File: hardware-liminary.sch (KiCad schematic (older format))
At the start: 51 parts, among them J1 Conn_01x05, J2 Conn_01x03, J3 Conn_01x03, J4 Conn_02x05_Odd_Even, J5 Conn_01x02, J6 UFL Conn, K1 HL2-1CH-12S, Q1 CMBT3904, Q2 PT204-6C, Q3 CMBT2222A, SW1 SW_Push, U1 EESAMR34J18-V1_CT, U2 LD1117S33TR_SOT223, U6 MCP6001T-I_OT

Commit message: eesam34
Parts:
- removed J6: UFL Conn, symbol 1909763-1:1909763-1
- removed LED1: 12-22/G6R6C-A31/2C, symbol LED_12-22:12-22SURSYGC_S530-A2_TR8
- removed U1: EESAMR34J18-V1_CT, symbol EESAMR34:EESAMR34J18-V1_CT
- removed U6: MCP6001T-I_OT, symbol MCP6001T-I_OT:MCP6001T-I_OT
- added U1: EESAMR34J18-V1_CT, proyect_EESAMR34:EESAMR34, symbol proyect_EESAMR34J18-V1_CT:EESAMR34J18-V1_CT
- JP3, JP4: footprint (none) -> Resistor_SMD:R_1206_3216Metric_Pad1.42x1.75mm_HandSolder
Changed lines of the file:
@@
 	3100 1350 3100 1250
-$Comp
-L MCP6001T-I_OT:MCP6001T-I_OT U6
-U 1 1 5F764C68
-P 3550 3500
-F 0 "U6" H 4150 3350 50  0000 C CNN
-F 1 "MCP6001T-I_OT" H 4150 3250 50  0000 C CNN
-F 2 "" H 4600 3900 50  0001 L CNN
-F 3 "http://docs-emea.rs-online.com/webdocs/0dd1/0900766b80dd189c.pdf" H 4600 3800 50  0001 L CNN
-F 4 "Single 1.8V Op Amp, 1MHz, I temp" H 4600 3700 50  0001 L CNN "Description"
-F 5 "1.45" H 4600 3600 50  0001 L CNN "Height"
-F 6 "Microchip" H 4600 3500 50  0001 L CNN "Manufacturer_Name"
-F 7 "MCP6001T-I/OT" H 4600 3400 50  0001 L CNN "Manufacturer_Part_Number"
-F 8 "MCP6001T-I/OT" H 4600 3300 50  0001 L CNN "Arrow Part Number"
-F 9 "https://www.arrow.com/en/products/mcp6001t-iot/microchip-technology" H 4600 3200 50  0001 L CNN "Arrow Price/Stock"
-F 10 "579-MCP6001T-I/OT" H 4600 3100 50  0001 L CNN "Mouser Part Number"
-F 11 "https://www.mouser.co.uk/ProductDetail/Microchip-Technology/MCP6001T-I-OT?qs=Q%2Fw7XRh99iki9dglS7IqJg%3D%3D" H 4600 3000 50  0001 L CNN "Mouser Price/Stock"
-	1    3550 3500
-	-1   0    0    -1
-$EndComp
 $Comp
 L Device:R R7
@@
 Wire Notes Line
 	5800 2400 500  2400
-$Comp
-L EESAMR34:EESAMR34J18-V1_CT U1
-U 1 1 5F95A58C
-P 2000 6650
-F 0 "U1" H 2150 6700 50  0000 R CNN
-F 1 "EESAMR34J18-V1_CT" H 2500 6550 50  0000 R CNN
-F 2 "" H 2000 6650 50  0001 L BNN
-F 3 "" H 2000 6650 118 0001 C CNN
-	1    2000 6650
-	1    0    0    -1
-$EndComp
 $Comp
 L power:GNDD #PWR0103
@@
 	1800 7650 1800 8150
 $Comp
-L LED_12-22:12-22SURSYGC_S530-A2_TR8 LED1
-U 1 1 5F8C80DF
-P 4500 8150
-F 0 "LED1" H 5000 8415 50  0000 C CNN
-F 1 "12-22/G6R6C-A31/2C" H 5000 8324 50  0000 C CNN
-F 2 "" H 5350 8250 50  0001 L CNN
-F 3 "" H 5350 8150 50  0001 L CNN
-F 4 "" H 5350 8050 50  0001 L CNN "Description"
-F 5 "2.2" H 5350 7950 50  0001 L CNN "Height"
-F 6 "Everlight" H 5350 7850 50  0001 L CNN "Manufacturer_Name"
-F 7 "12-22SURSYGC/S530-A2/TR8" H 5350 7750 50  0001 L CNN "Manufacturer_Part_Number"
-F 8 "12-22SURSYGC/S530-A2/TR8" H 5350 7650 50  0001 L CNN "Arrow Part Number"
-F 9 "" H 5350 7550 50  0001 L CNN "Arrow Price/Stock"
-F 10 "638-1222SURSYGCA2TR8" H 5350 7450 50  0001 L CNN "Mouser Part Number"
-F 11 "https://www.mouser.com/Search/Refine.aspx?Keyword=638-1222SURSYGCA2TR8" H 5350 7350 50  0001 L CNN "Mouser Price/Stock"
-	1    4500 8150
-	-1   0    0    -1
-$EndComp
-$Comp
 L Device:R R11
 U 1 1 5F8CC602
@@
 Antenna
 $Comp
-L 1909763-1:1909763-1 J6
-U 1 1 5FA17C3E
-P 6900 6000
-F 0 "J6" H 7188 6040 50  0000 L CNN
-F 1 "UFL Conn" H 7188 5949 50  0000 L CNN
-F 2 "" H 6900 6000 50  0001 L BNN
-F 3 "1909763-1" H 6900 6000 50  0001 L BNN
-F 4 "1" H 6900 6000 50  0001 L BNN "Field4"
-	1    6900 6000
-	1    0    0    -1
-$EndComp
-$Comp
 L power:GNDD #PWR014
 U 1 1 5FA23786
@@
 F 0 "JP4" H 6400 6164 50  0000 C CNN
 F 1 "Jumper" H 6400 6073 50  0000 C CNN
-F 2 "" H 6400 5900 50  0001 C CNN
+F 2 "Resistor_SMD:R_1206_3216Metric_Pad1.42x1.75mm_HandSolder" H 6400 5900 50  0001 C CNN
 F 3 "~" H 6400 5900 50  0001 C CNN
 	1    6400 5900
@@
 F 0 "JP3" H 6400 5814 50  0000 C CNN
 F 1 "Jumper" H 6400 5723 50  0000 C CNN
-F 2 "" H 6400 5550 50  0001 C CNN
+F 2 "Resistor_SMD:R_1206_3216Metric_Pad1.42x1.75mm_HandSolder" H 6400 5550 50  0001 C CNN
 F 3 "~" H 6400 5550 50  0001 C CNN
 	1    6400 5550
@@
 Wire Notes Line
 	7750 2350 7750 500
+$Comp
+L proyect_EESAMR34J18-V1_CT:EESAMR34J18-V1_CT U1
+U 1 1 5F767C93
+P 2000 6650
+F 0 "U1" H 1057 6646 50  0000 R CNN
+F 1 "EESAMR34J18-V1_CT" H 1057 6555 50  0000 R CNN
+F 2 "proyect_EESAMR34:EESAMR34" H 2000 6650 50  0001 L BNN
+F 3 "" H 2000 6650 50  0001 C CNN
+	1    2000 6650
+	1    0    0    -1
+$EndComp
 $EndSCHEMATC

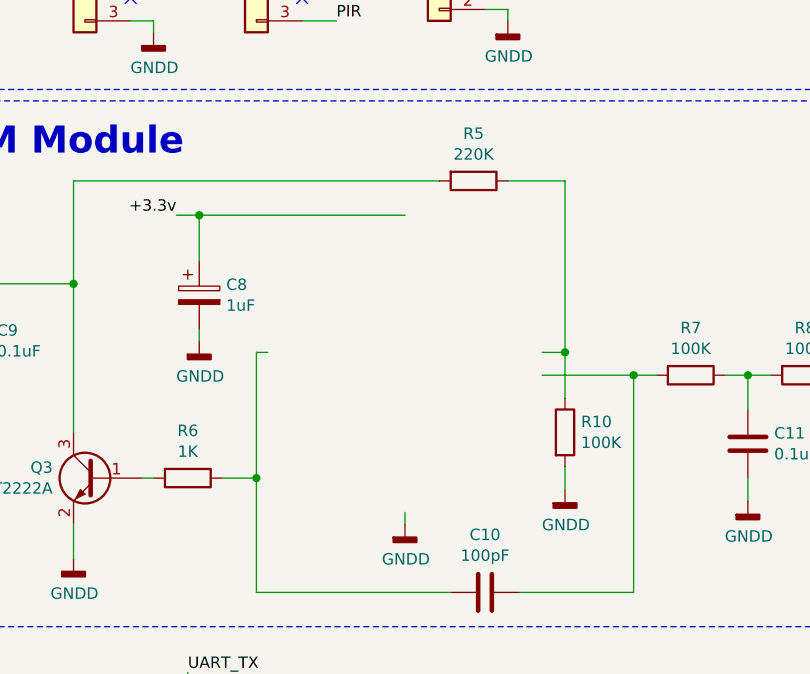
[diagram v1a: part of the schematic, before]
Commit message: opAmp
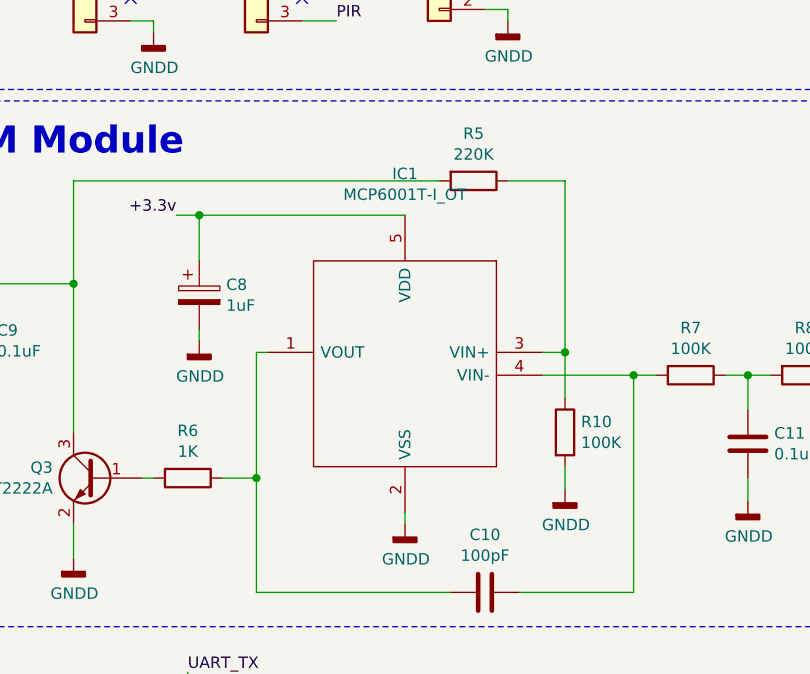
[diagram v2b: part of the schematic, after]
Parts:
- added IC1: MCP6001T-I_OT, proyect_MCP6001T-I_OT:SOT95P270X145-5N, symbol proyect_MCP6001T-I_OT:MCP6001T-I_OT
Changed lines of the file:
@@
 	1    0    0    -1
 $EndComp
+$Comp
+L proyect_MCP6001T-I_OT:MCP6001T-I_OT IC1
+U 1 1 5F79C962
+P 3550 3500
+F 0 "IC1" H 4150 4281 50  0000 C CNN
+F 1 "MCP6001T-I_OT" H 4150 4190 50  0000 C CNN
+F 2 "proyect_MCP6001T-I_OT:SOT95P270X145-5N" H 4600 3900 50  0001 L CNN
+F 3 "http://docs-emea.rs-online.com/webdocs/0dd1/0900766b80dd189c.pdf" H 4600 3800 50  0001 L CNN
+F 4 "Single 1.8V Op Amp, 1MHz, I temp" H 4600 3700 50  0001 L CNN "Description"
+F 5 "1.45" H 4600 3600 50  0001 L CNN "Height"
+F 6 "Microchip" H 4600 3500 50  0001 L CNN "Manufacturer_Name"
+F 7 "MCP6001T-I/OT" H 4600 3400 50  0001 L CNN "Manufacturer_Part_Number"
+F 8 "MCP6001T-I/OT" H 4600 3300 50  0001 L CNN "Arrow Part Number"
+F 9 "https://www.arrow.com/en/products/mcp6001t-iot/microchip-technology" H 4600 3200 50  0001 L CNN "Arrow Price/Stock"
+F 10 "579-MCP6001T-I/OT" H 4600 3100 50  0001 L CNN "Mouser Part Number"
+F 11 "https://www.mouser.co.uk/ProductDetail/Microchip-Technology/MCP6001T-I-OT?qs=Q%2Fw7XRh99iki9dglS7IqJg%3D%3D" H 4600 3000 50  0001 L CNN "Mouser Price/Stock"
+	1    3550 3500
+	-1   0    0    -1
+$EndComp
 $EndSCHEMATC
